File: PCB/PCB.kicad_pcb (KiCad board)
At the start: 2 copper layers, 13.8 x 16 mm, 30 parts, among them J1 Conn_01x06_Pin, U1 TPS7B6933, U2 A7106, U4 STM32G031F6Px, Y1 16MHz

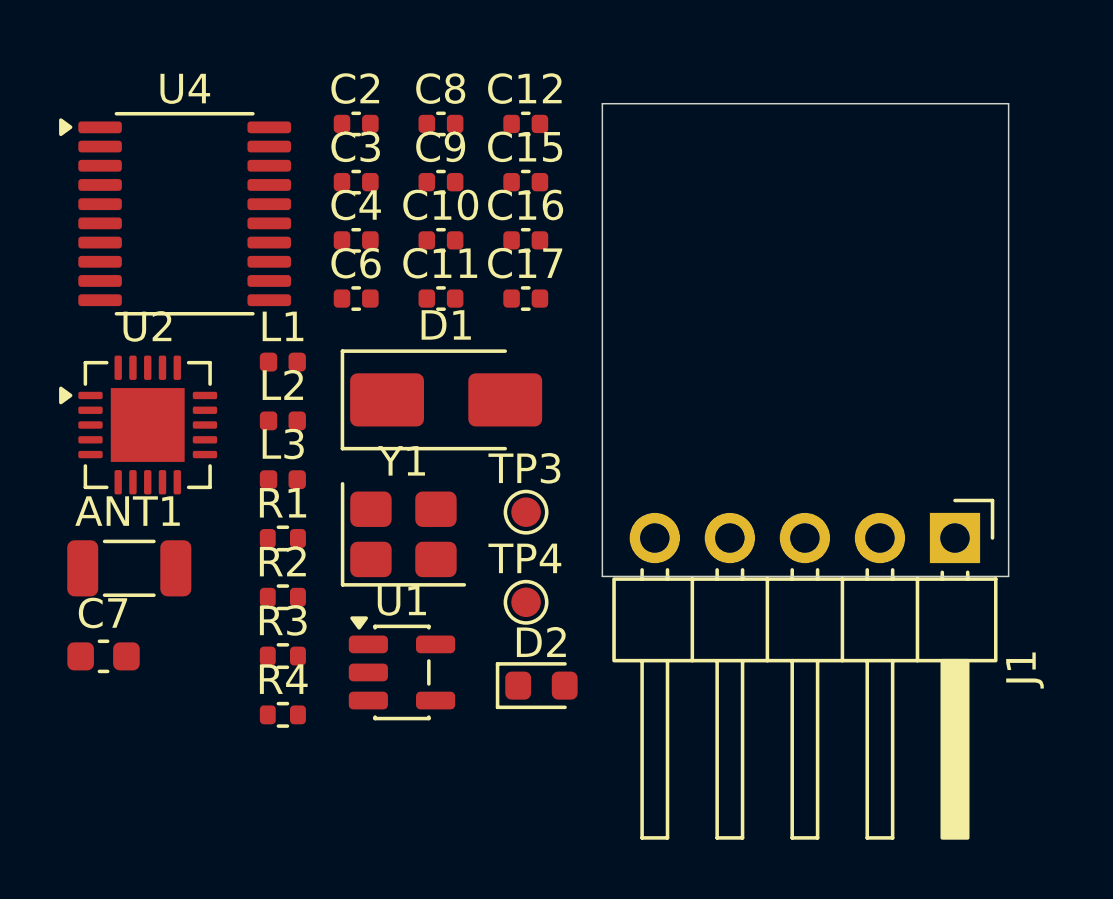
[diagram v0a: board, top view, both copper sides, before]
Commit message: Update public information and crystal
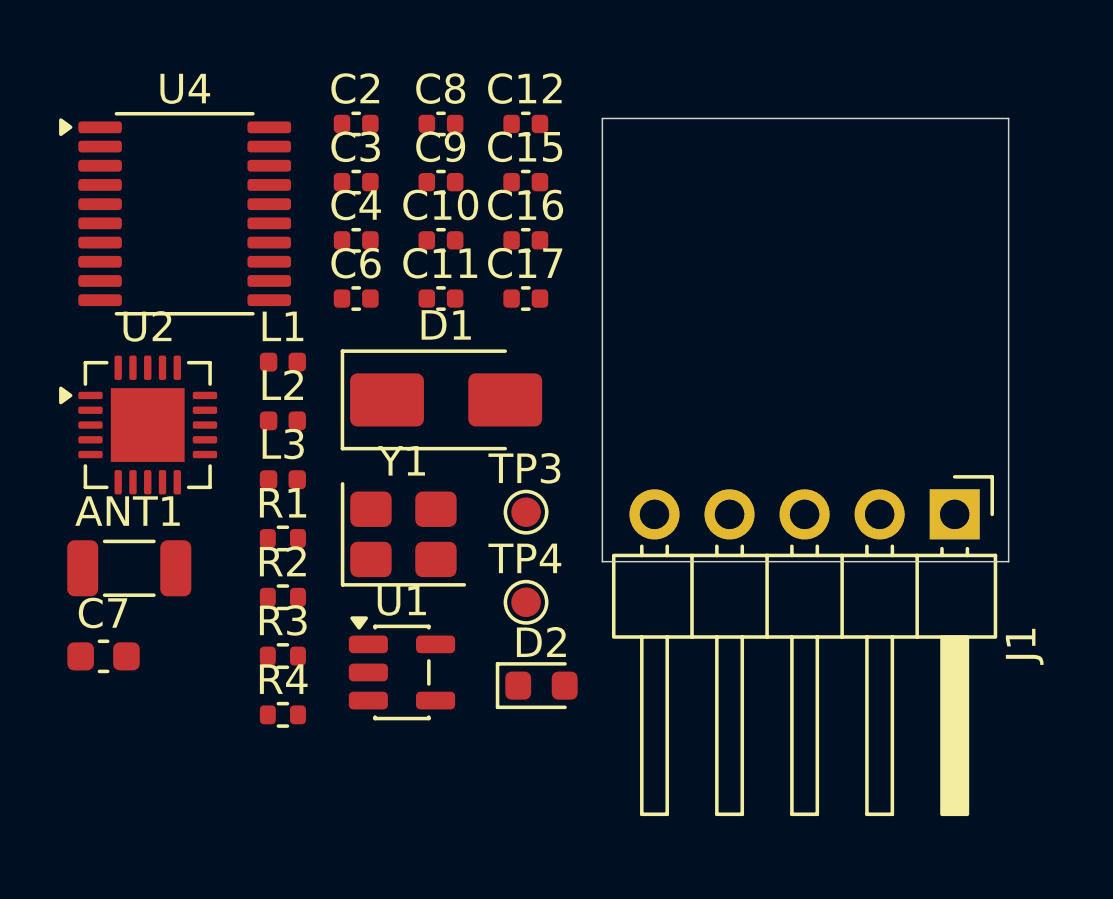
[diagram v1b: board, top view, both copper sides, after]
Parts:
- moved J1 0.80 mm to (188.9, 103.9)
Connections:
- J1 pad 1: GND -> /CH3
- J1 pad 2: Net-(D1-A2) -> /CH2
- J1 pad 4: /CH2 -> Net-(D1-A2)
- J1 pad 5: /CH3 -> GND
- Y1 pad 3: GND -> (no net)
- Y1 pad 4: GND -> (no net)
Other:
- board size 13.8 x 16 mm -> 13.8 x 15 mm
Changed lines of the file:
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@@
 	(footprint "Connector_PinHeader_2.54mm:PinHeader_1x05_P2.54mm_Horizontal"
 		(layer "F.Cu")
-		(at 188.96 104.7 -90)
+		(at 188.95 103.9 -90)
 		(descr "Through hole angled pin header, 1x05, 2.54mm pitch, 6mm pin length, single row")
 		(tags "Through hole angled pin header THT 1x05 2.54mm single row")
@@
 			(layers "*.Cu" "*.Mask")
 			(remove_unused_layers no)
-			(net "GND")
+			(net "/CH3")
 			(pinfunction "Pin_1_1")
 			(pintype "passive")
@@
 			(layers "*.Cu" "*.Mask")
 			(remove_unused_layers no)
-			(net "Net-(D1-A2)")
+			(net "/CH2")
 			(pinfunction "Pin_2_2")
 			(pintype "passive")
@@
 			(layers "*.Cu" "*.Mask")
 			(remove_unused_layers no)
-			(net "/CH2")
+			(net "Net-(D1-A2)")
 			(pinfunction "Pin_4_4")
 			(pintype "passive")
@@
 			(layers "*.Cu" "*.Mask")
 			(remove_unused_layers no)
-			(net "/CH3")
+			(net "GND")
 			(pinfunction "Pin_5_5")
 			(pintype "passive")
@@
 			(layers "F.Cu" "F.Mask" "F.Paste")
 			(roundrect_rratio 0.208333)
-			(net "GND")
 		)
 		(pad "4" smd roundrect
@@
 			(layers "F.Cu" "F.Mask" "F.Paste")
 			(roundrect_rratio 0.208333)
-			(net "GND")
 		)
 		(embedded_fonts no)
@@
 	)
 	(gr_rect
-		(start 177.025 90)
-		(end 190.775 106)
+		(start 177.025 90.5)
+		(end 190.775 105.5)
 		(stroke
 			(width 0.05)
